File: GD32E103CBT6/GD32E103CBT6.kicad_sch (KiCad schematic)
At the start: 15 parts

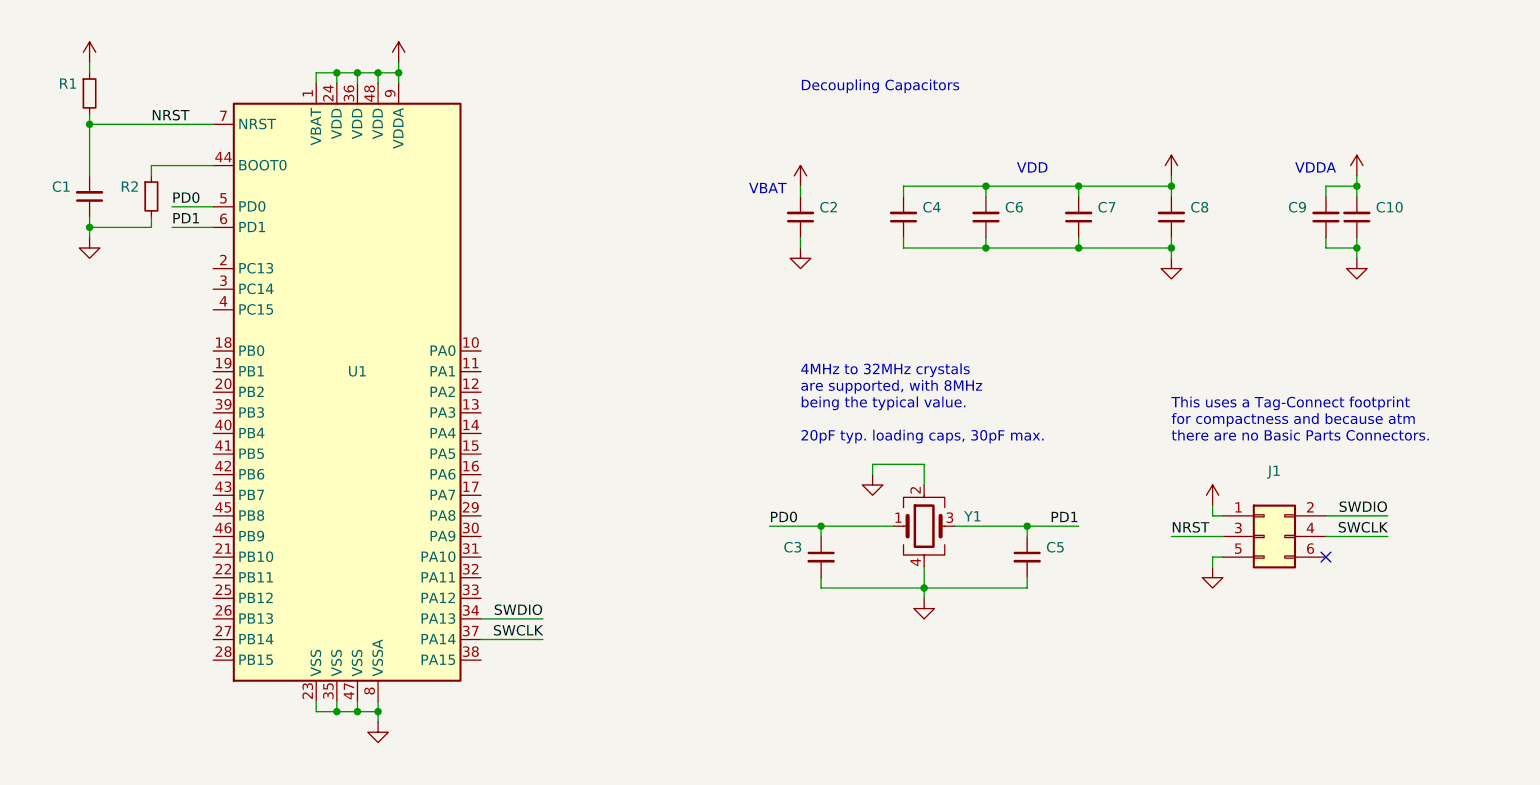
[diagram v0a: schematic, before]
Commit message: Reapply "Update modules to kicad v7 format"
This reverts commit fa5cc85431189ac7a3beedf0871b5723203ae43f.
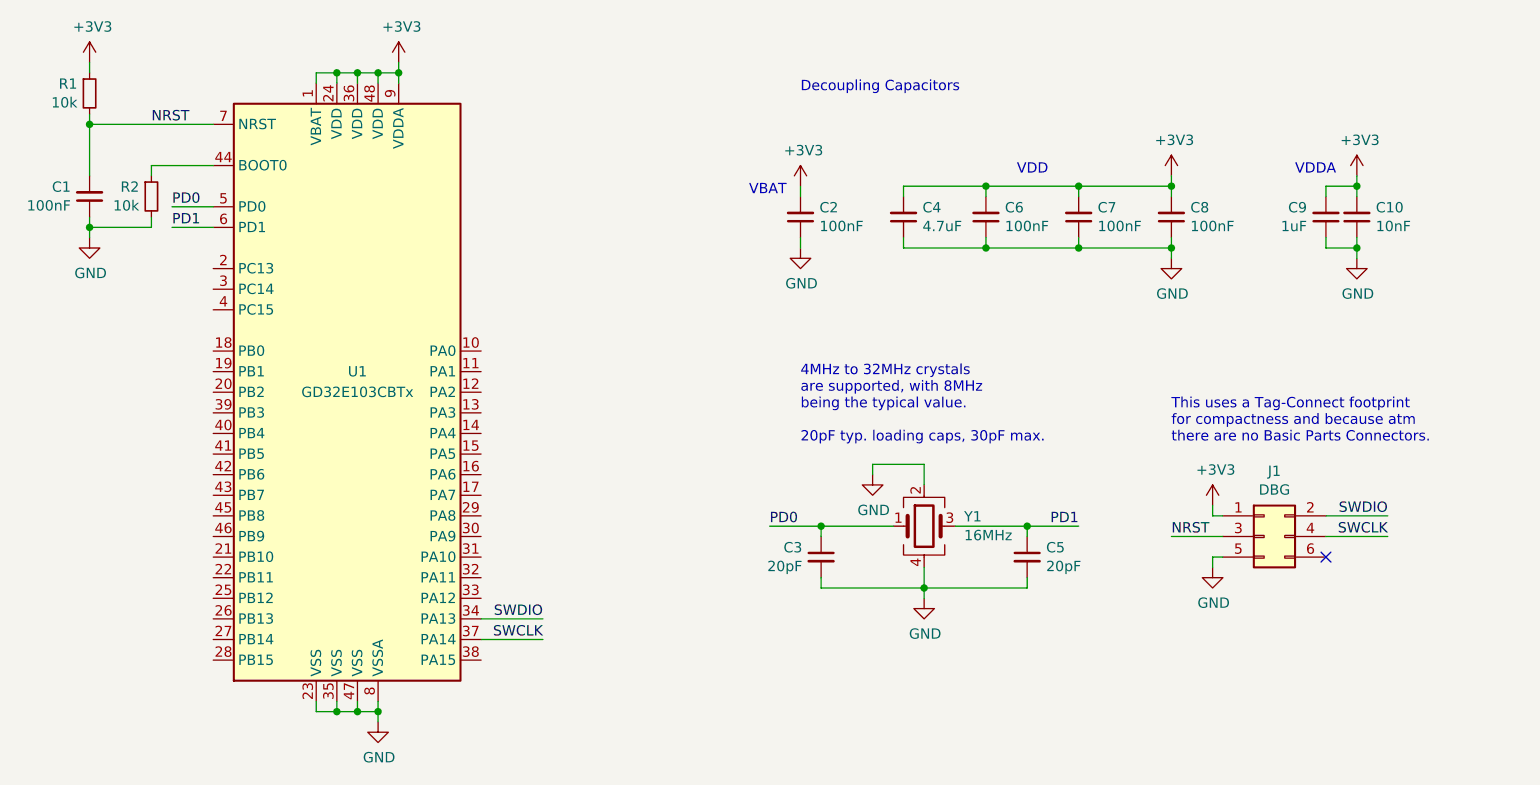
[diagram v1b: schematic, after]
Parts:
- C1, C2, C6, C7, C8: value (none) -> 100nF; footprint (none) -> Capacitor_SMD:C_0402_1005Metric
- C10: value (none) -> 10nF; footprint (none) -> Capacitor_SMD:C_0402_1005Metric
- C3, C5: value (none) -> 20pF; footprint (none) -> Capacitor_SMD:C_0402_1005Metric
- C4: value (none) -> 4.7uF; footprint (none) -> Capacitor_SMD:C_0402_1005Metric
- C9: value (none) -> 1uF; footprint (none) -> Capacitor_SMD:C_0402_1005Metric
- J1: value (none) -> DBG; footprint (none) -> Connector:Tag-Connect_TC2030-IDC-NL_2x03_P1.27mm_Vertical
- R1, R2: value (none) -> 10k; footprint (none) -> Resistor_SMD:R_0402_1005Metric
- U1: value (none) -> GD32E103CBTx; footprint (none) -> Package_QFP:LQFP-48_7x7mm_P0.5mm
- Y1: value (none) -> 16MHz; footprint (none) -> Crystal:Crystal_SMD_3225-4Pin_3.2x2.5mm
